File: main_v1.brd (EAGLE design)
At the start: 160 x 84.8 mm, 41 parts, among them IC1 MEGA8-P, IC2 7805TV

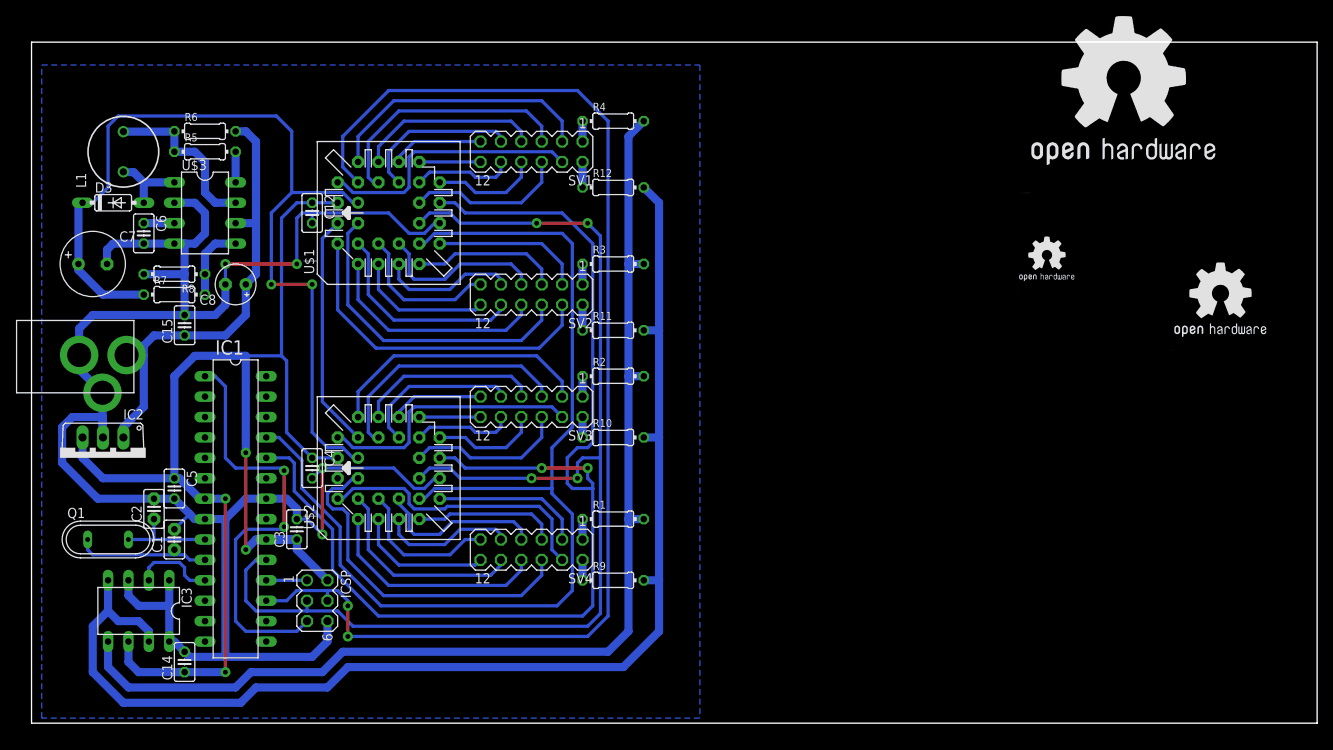
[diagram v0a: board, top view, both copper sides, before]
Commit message: Prettify
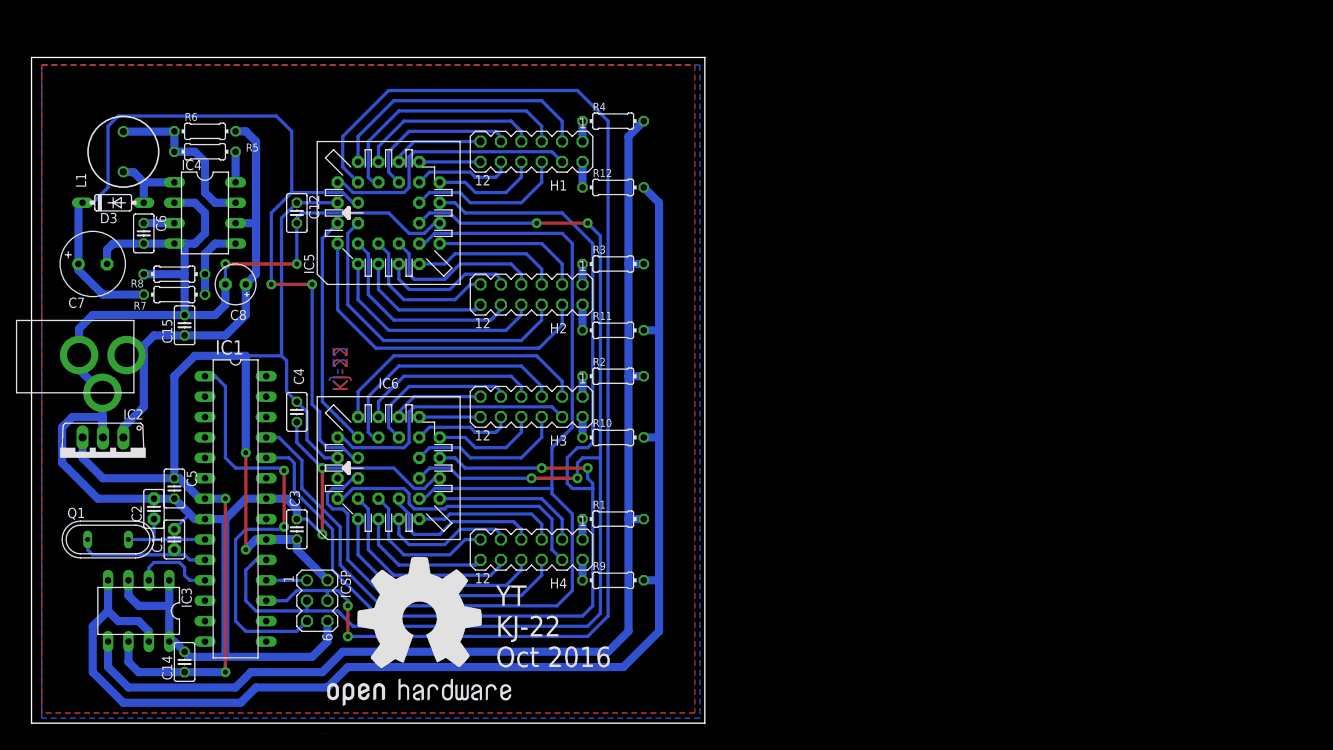
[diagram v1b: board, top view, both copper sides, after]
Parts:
- removed GOLD_ORB_SM2: OSHWLOGO_GOLD_ORB_MED, bfl:OSHW1
- removed GOLD_ORB_SM3: OSHWLOGO_GOLD_ORB_SM, bfl:OSHW2
- moved GOLD_ORB_SM1 110.5 mm to (35.6, -1.27)
- moved C4 7.24 mm to (33.0, 38.7)
- moved C12 1.90 mm to (33.0, 63.5)
- renumbered SV1 to H1, SV2 to H2, SV3 to H3, SV4 to H4, U$1 to IC5, U$2 to IC6, U$3 to IC4
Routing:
- net GND: track 247.0 -> 250.9 mm
- net VCC: track 170.1 -> 169.1 mm
- added copper zone on layer 1, net GND
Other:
- board size 160 x 84.8 mm -> 83.8 x 82.9 mm
- board text added: "KJ-22"
- board text added: "YT KJ-22 Oct 2016"
